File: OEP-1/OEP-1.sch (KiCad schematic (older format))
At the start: 33 parts, among them X1 Клеммник_х6, X2 Клеммник_х6, X3 Контрольная_точка_сопряжения, X4 Крепежное_отверстие_М3, X5 Крепежное_отверстие_М3, X6 Крепежное_отверстие_М3, X7 Крепежное_отверстие_М3

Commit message: ОУ заменен на транзисторный каскад (50х30 мм)
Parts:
- removed DA1: ОУ_LMx58, N_DD:SO-8, symbol OEP-1-rescue:ОУ_LMx58-elements
- added C7: Конденсатор_К10-83-25В-0,1_мкФ+-20проц., N_RLC:Конденсатор_SMD_IEC_0805, symbol OEP-1-rescue:Конденсатор_К10-83-25В-0,1_мкФ+-20проц.-MOTOR_2020_components
- added R15, R16: Резистор_0,125Вт, N_RLC:Резистор_SMD_IEC_0805_0,125_Вт, symbol OEP-1-rescue:Резистор_0,125Вт-elements
- added VT3, VT5: Транзистор_2Т3130А9, N_VD_HL:Корпус_КТ-46, symbol elements_2020:Транзистор_2Т3130А9
- added VT4, VT6: Транзистор_2Т3129Г9, N_VD_HL:Корпус_КТ-46, symbol elements_2020:Транзистор_2Т3129Г9
- C1, C3, C4, C6: symbol MOTOR_2020_components:Конденсатор_К10-83-25В-0,1_мкФ+-20проц. -> OEP-1-rescue:Конденсатор_К10-83-25В-0,1_мкФ+-20проц.-MOTOR_2020_components
- C2: symbol MOTOR_2020_components:Конденсатор_К53-56А-32В-22_мкФ+-10проц. -> OEP-1-rescue:Конденсатор_К53-56А-32В-22_мкФ+-10проц.-MOTOR_2020_components
- C5: footprint MOTOR_RLC:Конденсатор_SMD_IEC_0805 -> N_RLC:Конденсатор_SMD_IEC_0805; symbol MOTOR_2020_components:Конденсатор_К10-83-25В-0,1_мкФ+-20проц. -> OEP-1-rescue:Конденсатор_К10-83-25В-0,1_мкФ+-20проц.-MOTOR_2020_components
- G1: symbol MOTOR_2020_components:Микросхема_интегральная_КФ1158ЕН501А -> OEP-1-rescue:Микросхема_интегральная_КФ1158ЕН501А-MOTOR_2020_components
- X3: symbol MOTOR_2020_components:Контрольная_точка_сопряжения -> OEP-1-rescue:Контрольная_точка_сопряжения-MOTOR_2020_components
- X4, X5, X6, X7: symbol MOTOR_2020_components:Крепежное_отверстие_М3 -> OEP-1-rescue:Крепежное_отверстие_М3-MOTOR_2020_components
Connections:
- net 5V: now also C7.1, VT3.3, VT5.3
- net GND: now also C7.2, VT4.3, VT6.3
- net RX-1: now also R16.2
- net RX-2: now also R15.2
- net at R7.1: now also VT5.2, VT6.2
- net at R6.2: now also VT3.2, VT4.2
- new net: R15.1, VT3.1, VT4.1
- new net: R16.1, VT5.1, VT6.1
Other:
- note added: "DD1"
- note added: "DD2"
- note added: "G1"
- moved on the sheet: C1, C2, C3, C4, C5, C6, G1, R6, R7

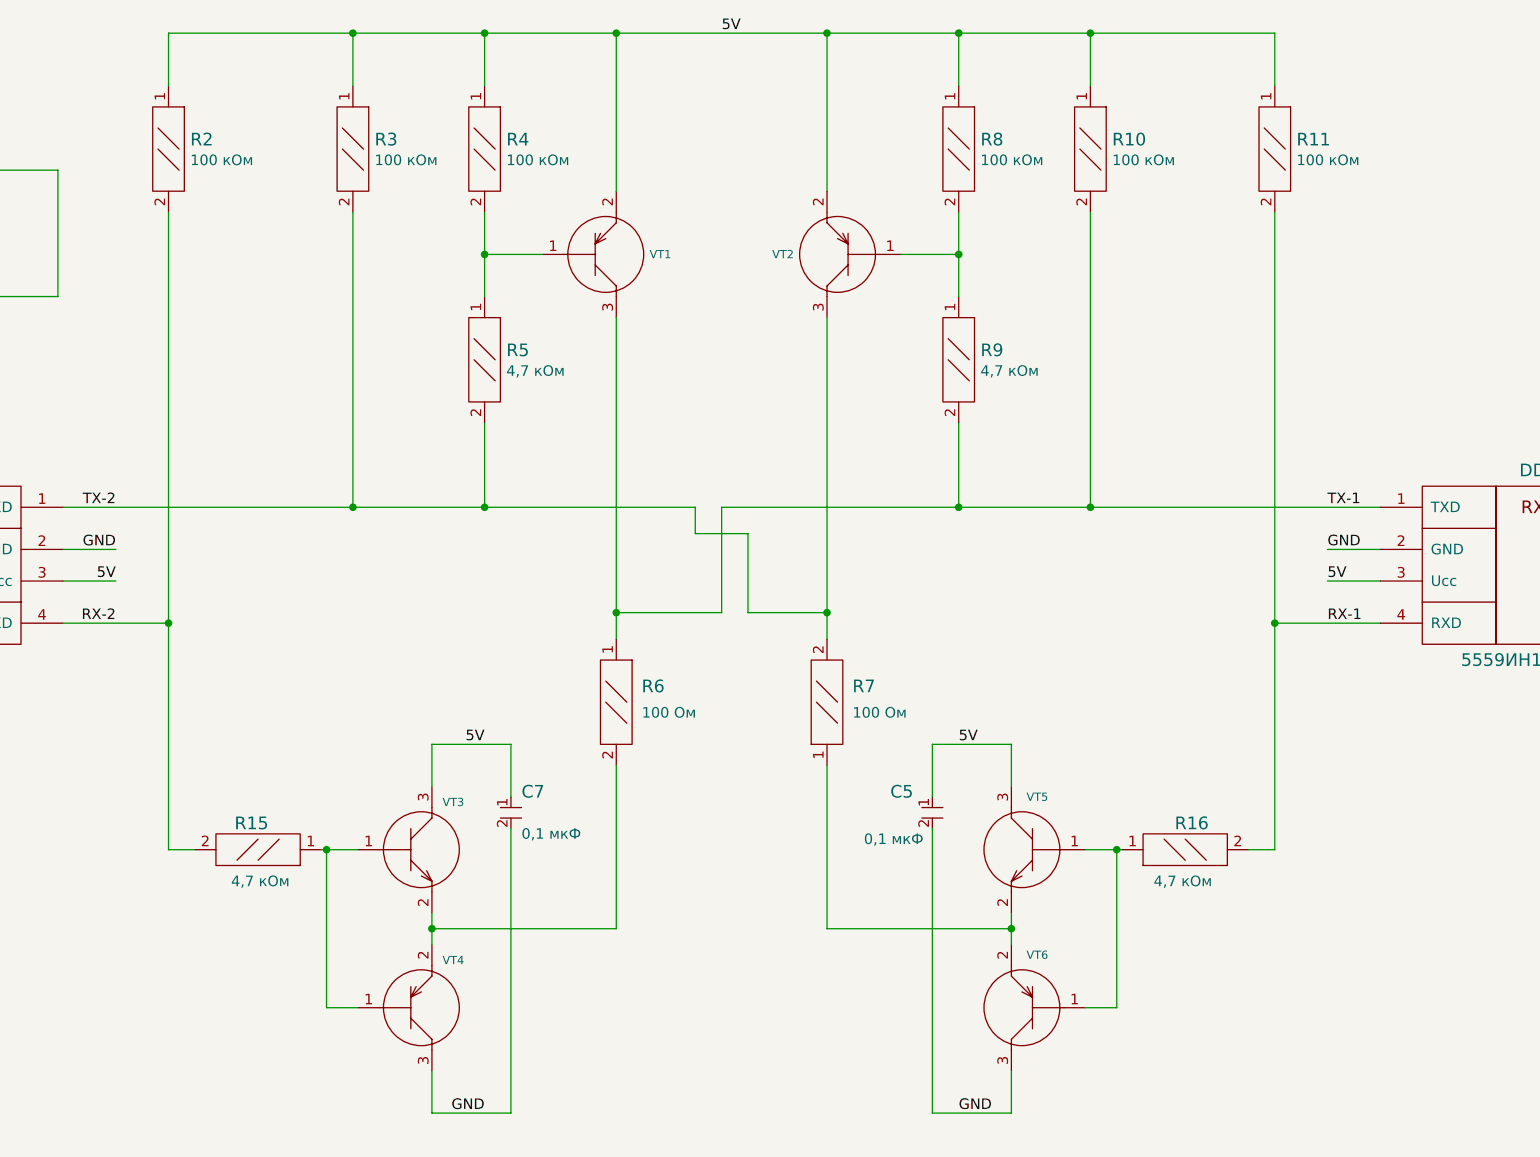
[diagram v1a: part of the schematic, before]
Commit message: причесана трассировка, добавлены gerber-файлы
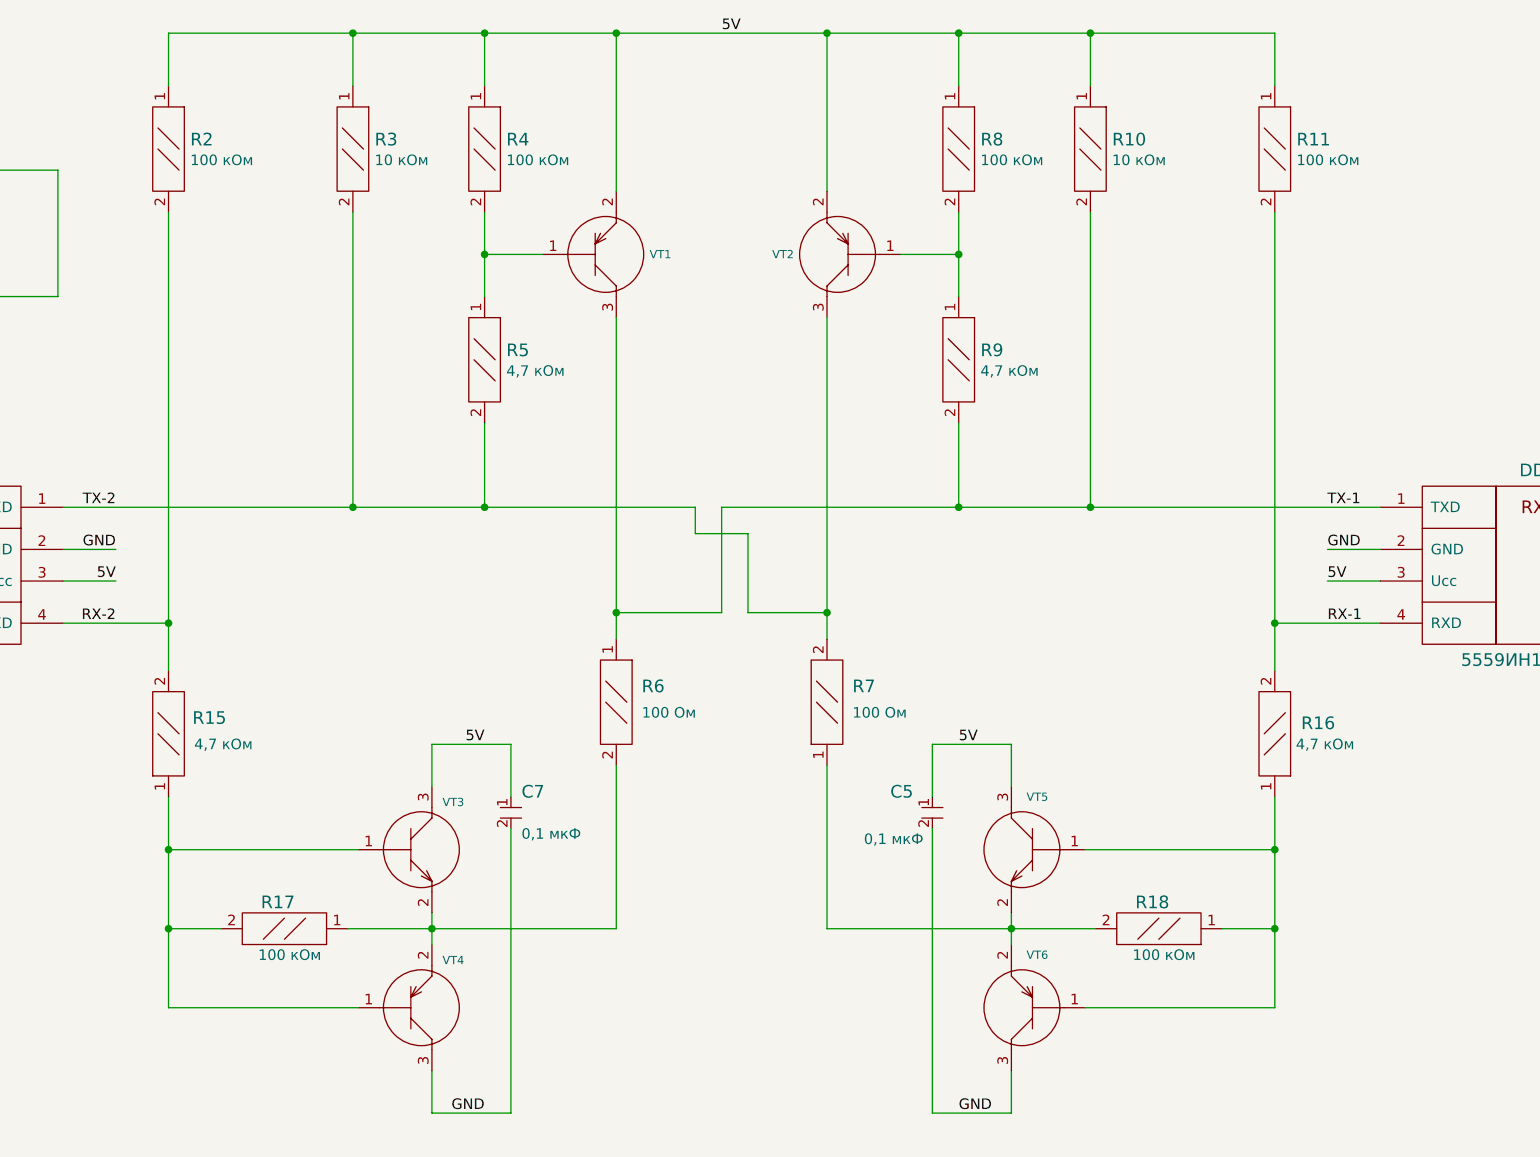
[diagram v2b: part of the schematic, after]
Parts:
- added R17, R18: Резистор_0,125Вт, N_RLC:Резистор_SMD_IEC_0805_0,125_Вт, symbol OEP-1-rescue:Резистор_0,125Вт-elements
- R10, R3: Номинал 100 кОм -> 10 кОм
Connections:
- net at R7.1, VT5.2, VT6.2: now also R18.2
- net at R6.2, VT3.2, VT4.2: now also R17.1
- net at R15.1, VT3.1, VT4.1: now also R17.2
- net at R16.1, VT5.1, VT6.1: now also R18.1
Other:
- moved on the sheet: R15, R16
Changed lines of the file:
@@
 F 2 "MOTOR_RLC:Резистор_SMD_IEC_0805_0,125_Вт" H 6125 2800 60  0001 C CNN
 F 3 "" H 6125 2800 60  0001 C CNN
-F 4 "100 кОм" V 6178 2903 50  0000 L CNN "Номинал"
+F 4 "10 кОм" V 6178 2903 50  0000 L CNN "Номинал"
 F 5 "R101" H 6125 2800 50  0001 C CNN "УГО"
 	1    6125 2800
@@
 F 2 "MOTOR_RLC:Резистор_SMD_IEC_0805_0,125_Вт" H 9625 2800 60  0001 C CNN
 F 3 "" H 9625 2800 60  0001 C CNN
-F 4 "100 кОм" V 9678 2903 50  0000 L CNN "Номинал"
+F 4 "10 кОм" V 9678 2903 50  0000 L CNN "Номинал"
 F 5 "R101" H 9625 2800 50  0001 C CNN "УГО"
 	1    9625 2800
@@
 Wire Wire Line
 	5250 5050 5250 3100
-Connection ~ 5250 5050
 $Comp
 L OEP-1-rescue:Резистор_0,125Вт-elements R11
@@
 Wire Wire Line
 	10500 3100 10500 5050
-Connection ~ 10500 5050
 $Comp
 L elements_2020:Транзистор_2Т3130А9 VT3
@@
 L OEP-1-rescue:Резистор_0,125Вт-elements R15
 U 1 1 60D75E73
-P 5675 6125
-F 0 "R15" H 5625 6000 60  0000 L CNN
-F 1 "Резистор_0,125Вт" H 5675 5975 60  0001 C CNN
-F 2 "N_RLC:Резистор_SMD_IEC_0805_0,125_Вт" H 5675 6125 60  0001 C CNN
-F 3 "" H 5675 6125 60  0001 C CNN
-F 4 "4,7 кОм" H 5525 6275 50  0000 L CNN "Номинал"
-F 5 "R101" H 5675 6125 50  0001 C CNN "УГО"
-	1    5675 6125
-	-1   0    0    1
+P 5250 5575
+F 0 "R15" V 5325 5300 60  0000 L CNN
+F 1 "Резистор_0,125Вт" H 5250 5425 60  0001 C CNN
+F 2 "N_RLC:Резистор_SMD_IEC_0805_0,125_Вт" H 5250 5575 60  0001 C CNN
+F 3 "" H 5250 5575 60  0001 C CNN
+F 4 "4,7 кОм" V 5200 5175 50  0000 L CNN "Номинал"
+F 5 "R101" H 5250 5575 50  0001 C CNN "УГО"
+	1    5250 5575
+	0    -1   -1   0
 $EndComp
 Wire Wire Line
@@
 Wire Wire Line
 	8375 3600 8375 5000
-Wire Wire Line
-	5375 6125 5250 6125
 Text Notes 12700 7950 0    50   ~ 0
 DD1
@@
 L OEP-1-rescue:Резистор_0,125Вт-elements R16
 U 1 1 60DD88BA
-P 10075 6125
-F 0 "R16" H 10025 6000 60  0000 L CNN
-F 1 "Резистор_0,125Вт" H 10075 5975 60  0001 C CNN
-F 2 "N_RLC:Резистор_SMD_IEC_0805_0,125_Вт" H 10075 6125 60  0001 C CNN
-F 3 "" H 10075 6125 60  0001 C CNN
-F 4 "4,7 кОм" H 9925 6275 50  0000 L CNN "Номинал"
-F 5 "R101" H 10075 6125 50  0001 C CNN "УГО"
-	1    10075 6125
-	1    0    0    1
+P 10500 5575
+F 0 "R16" V 10550 5700 60  0000 L CNN
+F 1 "Резистор_0,125Вт" H 10500 5425 60  0001 C CNN
+F 2 "N_RLC:Резистор_SMD_IEC_0805_0,125_Вт" H 10500 5575 60  0001 C CNN
+F 3 "" H 10500 5575 60  0001 C CNN
+F 4 "4,7 кОм" V 10450 5675 50  0000 L CNN "Номинал"
+F 5 "R101" H 10500 5575 50  0001 C CNN "УГО"
+	1    10500 5575
+	0    1    -1   0
 $EndComp
 Wire Wire Line
@@
 	8375 5725 8375 6500
 Wire Wire Line
-	5250 5050 5250 6125
-Wire Wire Line
-	10375 6125 10500 6125
-Wire Wire Line
-	10500 6125 10500 5050
-Wire Wire Line
-	5975 6125 6000 6125
-Wire Wire Line
 	6500 6500 7375 6500
 Wire Wire Line
 	8375 6500 9250 6500
 Wire Wire Line
-	9775 6125 9750 6125
-Wire Wire Line
-	9750 6125 9750 6875
-Wire Wire Line
-	9750 6875 9600 6875
-Connection ~ 9750 6125
-Wire Wire Line
-	9750 6125 9600 6125
-Wire Wire Line
-	6000 6125 6000 6875
-Wire Wire Line
-	6000 6875 6150 6875
-Connection ~ 6000 6125
-Wire Wire Line
-	6000 6125 6150 6125
+	10500 6125 10500 6500
+Wire Wire Line
+	5250 6125 5250 6500
+$Comp
+L OEP-1-rescue:Резистор_0,125Вт-elements R17
+U 1 1 60D3544A
+P 5800 6500
+F 0 "R17" H 5750 6375 60  0000 L CNN
+F 1 "Резистор_0,125Вт" H 5800 6350 60  0001 C CNN
+F 2 "N_RLC:Резистор_SMD_IEC_0805_0,125_Вт" H 5800 6500 60  0001 C CNN
+F 3 "" H 5800 6500 60  0001 C CNN
+F 4 "100 кОм" H 5625 6625 50  0000 L CNN "Номинал"
+F 5 "R101" H 5800 6500 50  0001 C CNN "УГО"
+	1    5800 6500
+	-1   0    0    1
+$EndComp
+Wire Wire Line
+	5250 5050 5250 5275
+Connection ~ 5250 5050
+Wire Wire Line
+	5250 5875 5250 6125
+Connection ~ 5250 6125
+Wire Wire Line
+	5250 6125 6150 6125
+Wire Wire Line
+	5250 6875 6150 6875
+Wire Wire Line
+	6100 6500 6500 6500
+Wire Wire Line
+	5500 6500 5250 6500
+Connection ~ 5250 6500
+Wire Wire Line
+	5250 6500 5250 6875
+Wire Wire Line
+	10500 5050 10500 5275
+Connection ~ 10500 5050
+Wire Wire Line
+	10500 5875 10500 6125
+Connection ~ 10500 6125
+Wire Wire Line
+	9600 6125 10500 6125
+Wire Wire Line
+	9600 6875 10500 6875
+$Comp
+L OEP-1-rescue:Резистор_0,125Вт-elements R18
+U 1 1 60D7F7C1
+P 9950 6500
+F 0 "R18" H 9900 6375 60  0000 L CNN
+F 1 "Резистор_0,125Вт" H 9950 6350 60  0001 C CNN
+F 2 "N_RLC:Резистор_SMD_IEC_0805_0,125_Вт" H 9950 6500 60  0001 C CNN
+F 3 "" H 9950 6500 60  0001 C CNN
+F 4 "100 кОм" H 9775 6625 50  0000 L CNN "Номинал"
+F 5 "R101" H 9950 6500 50  0001 C CNN "УГО"
+	1    9950 6500
+	-1   0    0    1
+$EndComp
+Wire Wire Line
+	10250 6500 10500 6500
+Connection ~ 10500 6500
+Wire Wire Line
+	10500 6500 10500 6875
+Wire Wire Line
+	9650 6500 9250 6500
 $EndSCHEMATC
